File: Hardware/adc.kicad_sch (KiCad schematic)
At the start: 18 parts, among them U2 ADS1256IDBT, Y1 8MHz

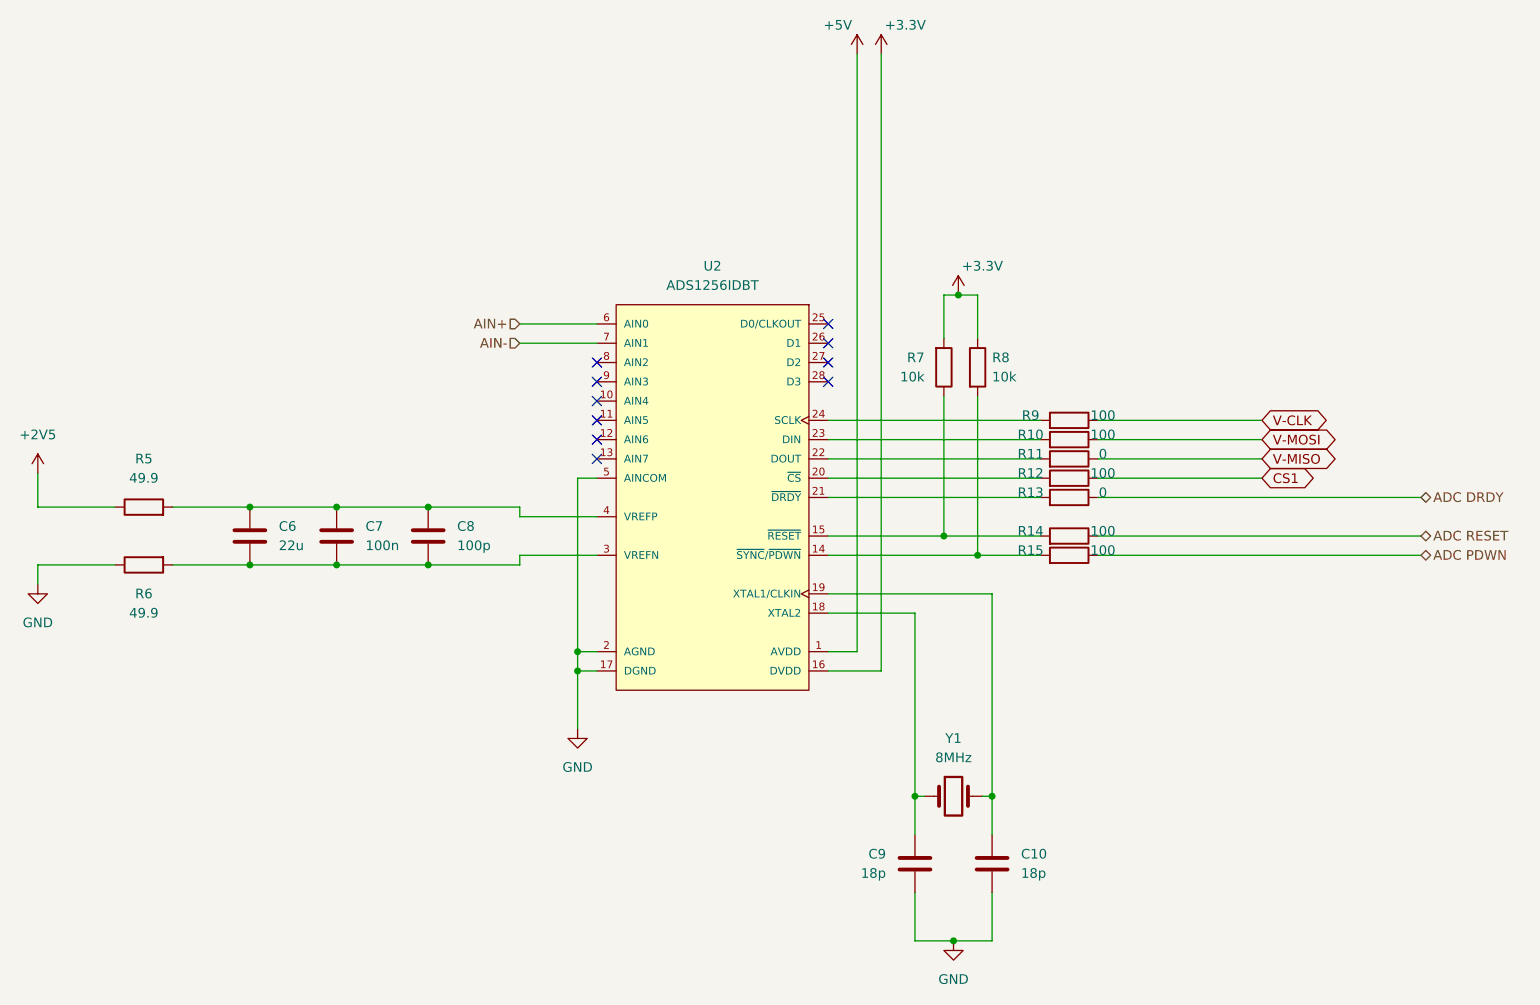
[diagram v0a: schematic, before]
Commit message: Version 0.1
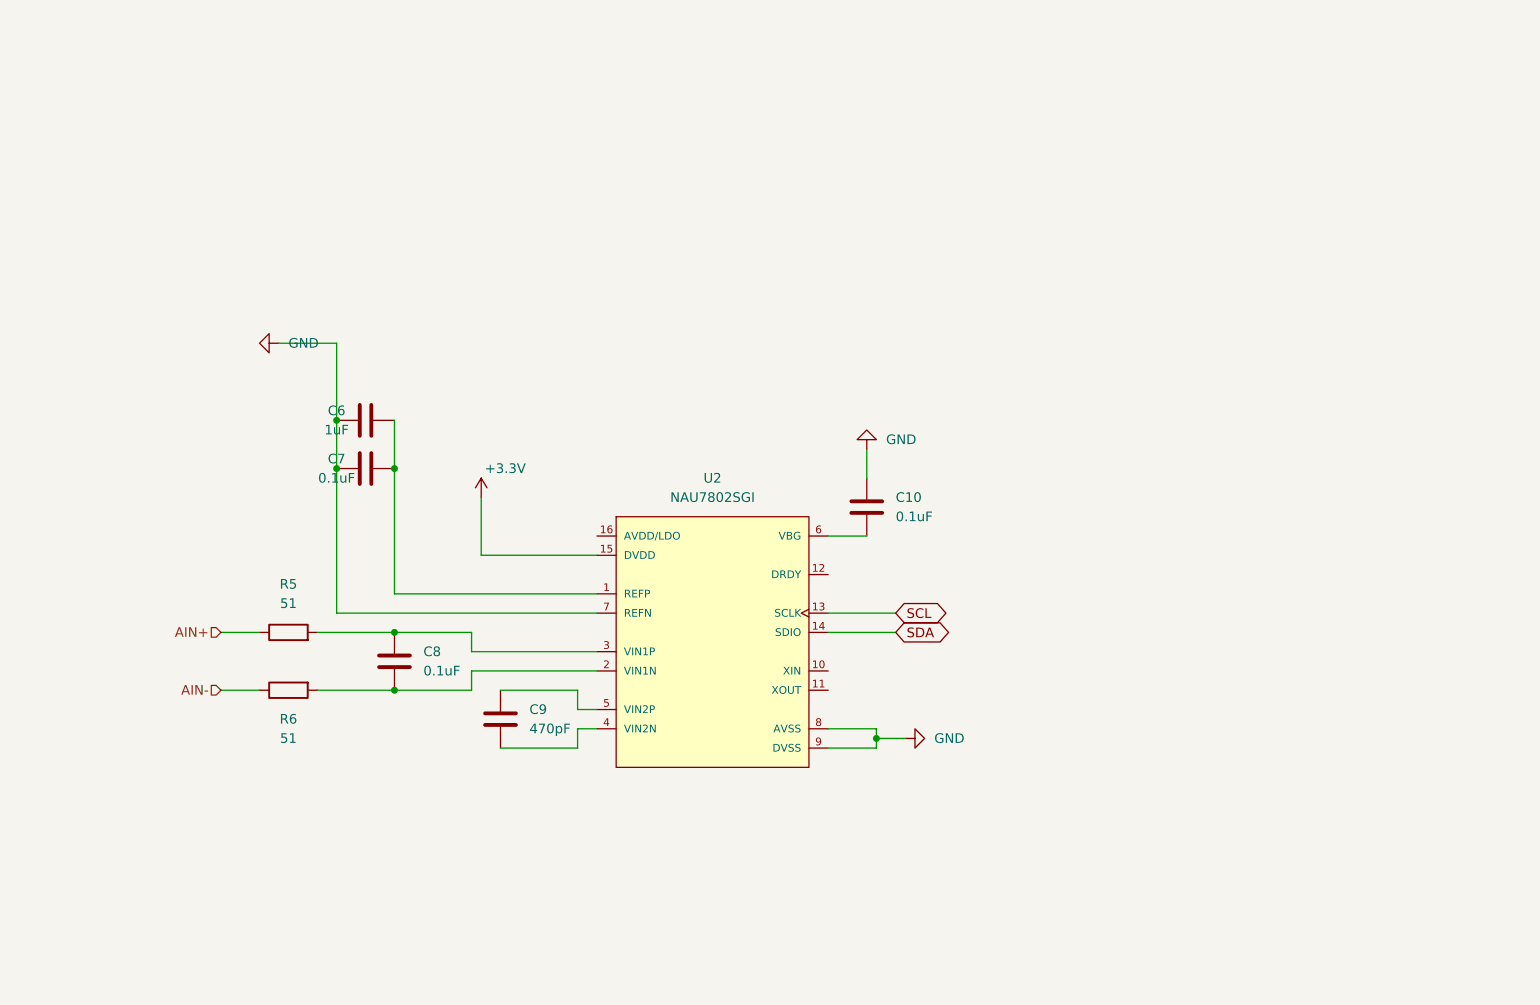
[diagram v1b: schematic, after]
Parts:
- removed R10, R12, R14, R15, R9: 100, Resistor_SMD:R_0805_2012Metric_Pad1.20x1.40mm_HandSolder, symbol Device:R
- removed R11, R13: 0, Resistor_SMD:R_0805_2012Metric_Pad1.20x1.40mm_HandSolder, symbol Device:R
- removed R7, R8: 10k, Resistor_SMD:R_0805_2012Metric_Pad1.20x1.40mm_HandSolder, symbol Device:R
- removed U2: ADS1256IDBT, ADS1256IDBT:SOP65P780X200-28N, symbol ADS1256:ADS1256IDBT
- removed Y1: 8MHz, Crystal:Crystal_SMD_3225-4Pin_3.2x2.5mm_HandSoldering, symbol Device:Crystal
- added U2: NAU7802SGI, symbol Nuvoton_-_NAU7802SGI:NAU7802SGI
- C10: value 18p -> 0.1uF; footprint Capacitor_SMD:C_0805_2012Metric_Pad1.18x1.45mm_HandSolder -> Capacitor_SMD:C_0603_1608Metric_Pad1.08x0.95mm_HandSolder
- C6: value 22u -> 1uF; footprint Capacitor_SMD:C_0805_2012Metric_Pad1.18x1.45mm_HandSolder -> Capacitor_SMD:C_0603_1608Metric_Pad1.08x0.95mm_HandSolder
- C7: value 100n -> 0.1uF; footprint Capacitor_SMD:C_0805_2012Metric_Pad1.18x1.45mm_HandSolder -> Capacitor_SMD:C_0603_1608Metric_Pad1.08x0.95mm_HandSolder
- C8: value 100p -> 0.1uF; footprint Capacitor_SMD:C_0805_2012Metric_Pad1.18x1.45mm_HandSolder -> Capacitor_SMD:C_0603_1608Metric_Pad1.08x0.95mm_HandSolder
- C9: value 18p -> 470pF; footprint Capacitor_SMD:C_0805_2012Metric_Pad1.18x1.45mm_HandSolder -> Capacitor_SMD:C_0603_1608Metric_Pad1.08x0.95mm_HandSolder
- R5, R6: value 49.9 -> 51; footprint Resistor_SMD:R_0805_2012Metric_Pad1.20x1.40mm_HandSolder -> Resistor_SMD:R_0603_1608Metric_Pad0.98x0.95mm_HandSolder
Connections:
- net +2V5 is gone; now on net AIN+: R5.1
- net +3V3: now also U2.15 (DVDD)
- net AIN-: now also R6.1
- net GND: now also C10.1, C6.1, C7.1, U2.7 (REFN), U2.8 (AVSS), U2.9 (DVSS); no longer C10.2, C9.1, R6.1
- net at C8.1, R5.2: now also U2.3 (VIN1P); no longer C6.1, C7.1
- net at C9.2: now also U2.4 (VIN2N)
- net at C6.2, C7.2: now also U2.1 (REFP); no longer C8.2, R6.2
- new net: C10.2, U2.6 (VBG)
- new net: C8.2, R6.2, U2.2 (VIN1N)
- new net: C9.1, U2.5 (VIN2P)
- new net SCL: U2.13 (SCLK)
- new net SDA: U2.14 (SDIO)
- no-connect marks 10 -> 0
